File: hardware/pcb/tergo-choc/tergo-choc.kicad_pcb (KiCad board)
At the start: 2 copper layers, 87.7 x 67.9 mm, 43 parts, among them J1 TRRS_SOCKET, J12 Conn_01x01_Socket, J13 Conn_01x01_Socket, J14 Conn_01x01_Socket, J15 Conn_01x01_Socket, J18 Conn_01x01_Socket, J19 Conn_01x01_Socket, J2 Conn_01x04_Socket, J20 Conn_01x01_Socket, J21 Conn_01x01_Socket, J22 Conn_01x01_Socket, J23 Conn_01x01_Socket, J24 Conn_01x01_Socket, J25 Conn_01x01_Socket, J26 Conn_01x01_Socket, J27 Conn_01x01_Socket, J28 Conn_01x01_Socket, J29 Conn_01x01_Socket, J3 TRRS_SOCKET, J30 Conn_01x01_Socket, J31 Conn_01x01_Socket, J32 Conn_01x01_Socket, J33 Conn_01x01_Socket, J34 Conn_01x01_Socket, J35 Conn_01x01_Socket, SW1 RST_LEFT, SW30 RST_RIGHT, U1 Raspberry_Pi_Pico, U2 Raspberry_Pi_Pico

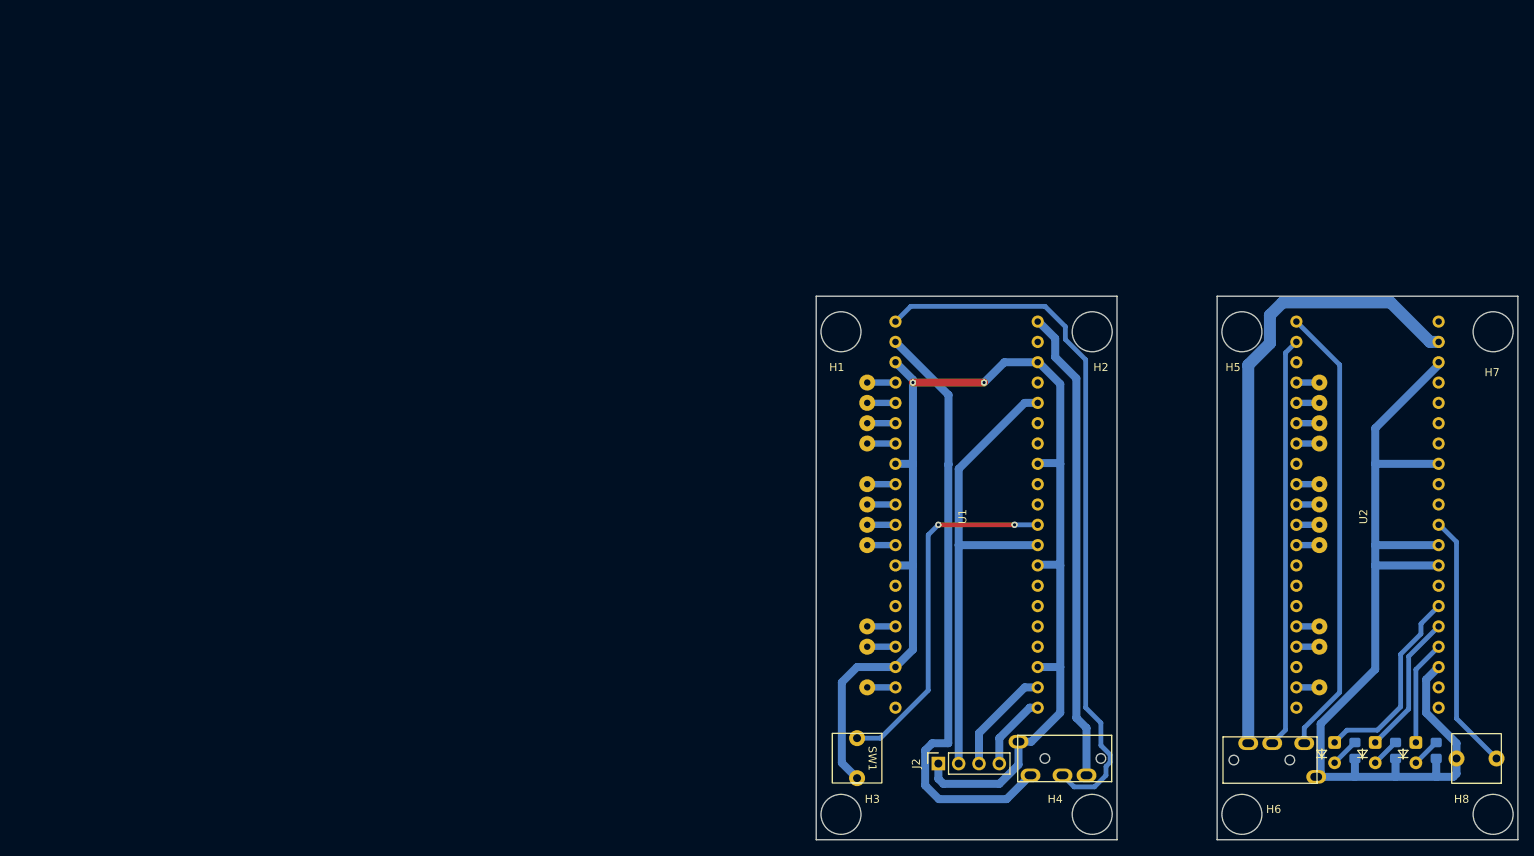
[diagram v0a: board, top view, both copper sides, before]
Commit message: win
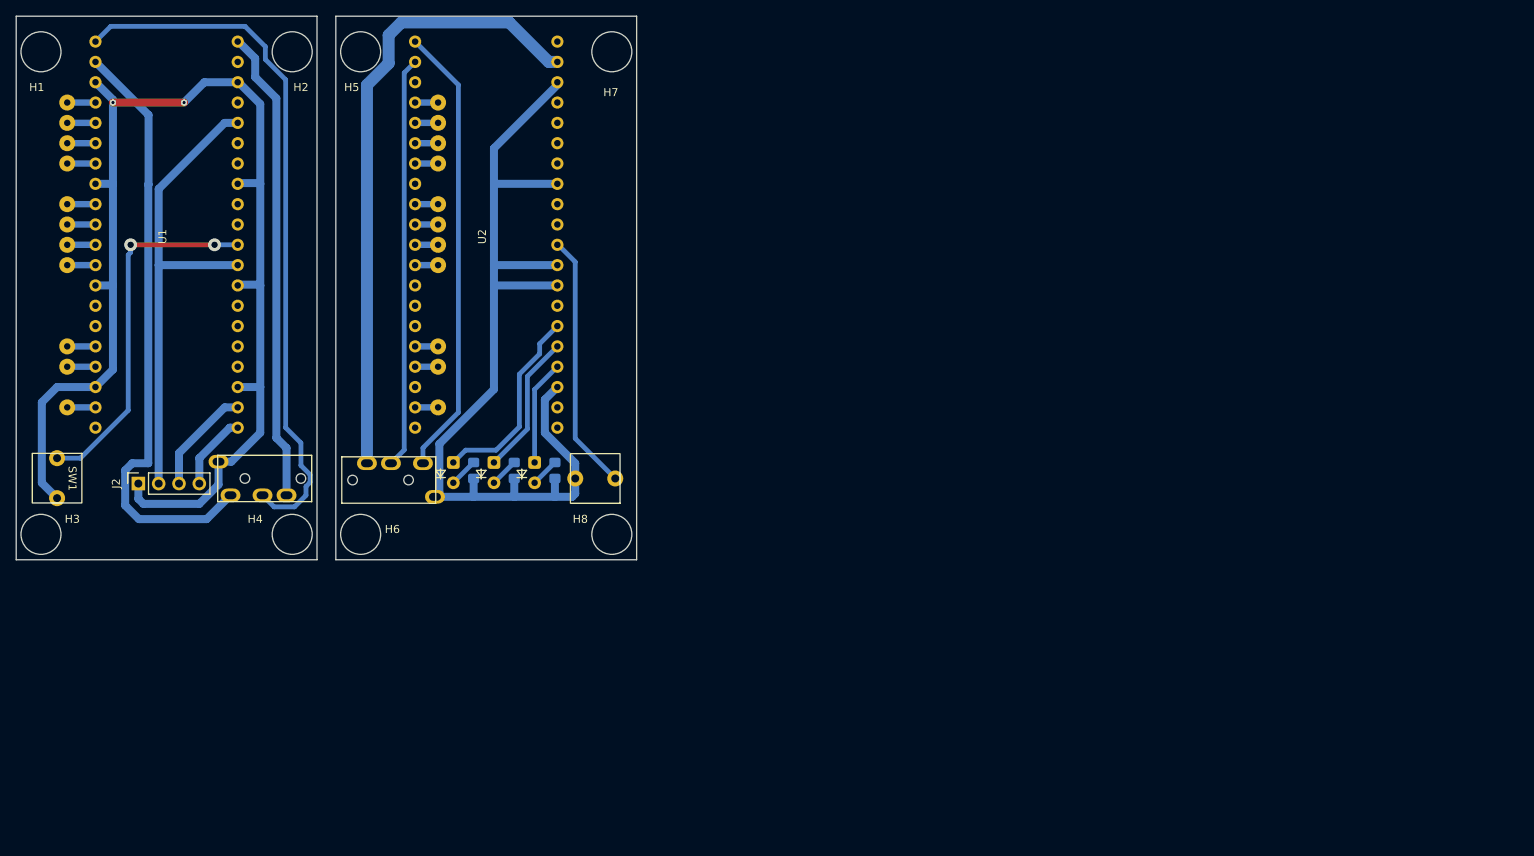
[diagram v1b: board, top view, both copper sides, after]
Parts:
- moved J27 115.6 mm to (69.5, 31.0)
- moved J34 115.6 mm to (69.5, 59.0)
- moved D10 115.6 mm to (71.5, 72.2)
- moved D60 115.6 mm to (81.6, 72.2)
- moved H7 115.6 mm to (91.3, 19.6)
- moved H8 115.6 mm to (91.3, 79.9)
- moved J25 115.6 mm to (69.5, 26.0)
- moved J26 115.6 mm to (69.5, 28.5)
- moved J28 115.6 mm to (69.5, 33.6)
- moved J29 115.6 mm to (69.5, 38.7)
- moved J30 115.6 mm to (69.5, 41.2)
- moved J31 115.6 mm to (69.5, 43.7)
- moved J32 115.6 mm to (69.5, 46.3)
- moved J33 115.6 mm to (69.5, 56.4)
- moved J35 115.6 mm to (69.5, 64.1)
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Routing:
- net /RST_L: track 45.0 -> 45.6 mm
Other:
- board size 87.7 x 67.9 mm -> 77.6 x 67.9 mm
